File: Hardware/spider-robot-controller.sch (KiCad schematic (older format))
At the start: 27 parts, among them CON1 AVR-ISP-6, CON2 BARREL_JACK, IC1 ATMEGA328-P, P1 SERVO_HEADER, P10 SERVO_HEADER, P11 SERVO_HEADER, P12 SERVO_HEADER, P13 Bluetooth_header, P2 SERVO_HEADER, P3 SERVO_HEADER, P4 SERVO_HEADER, P5 SERVO_HEADER, P6 SERVO_HEADER, P7 SERVO_HEADER, P8 SERVO_HEADER, P9 SERVO_HEADER, SW1 SW_PUSH, U1 LM7805, Y1 16MHz

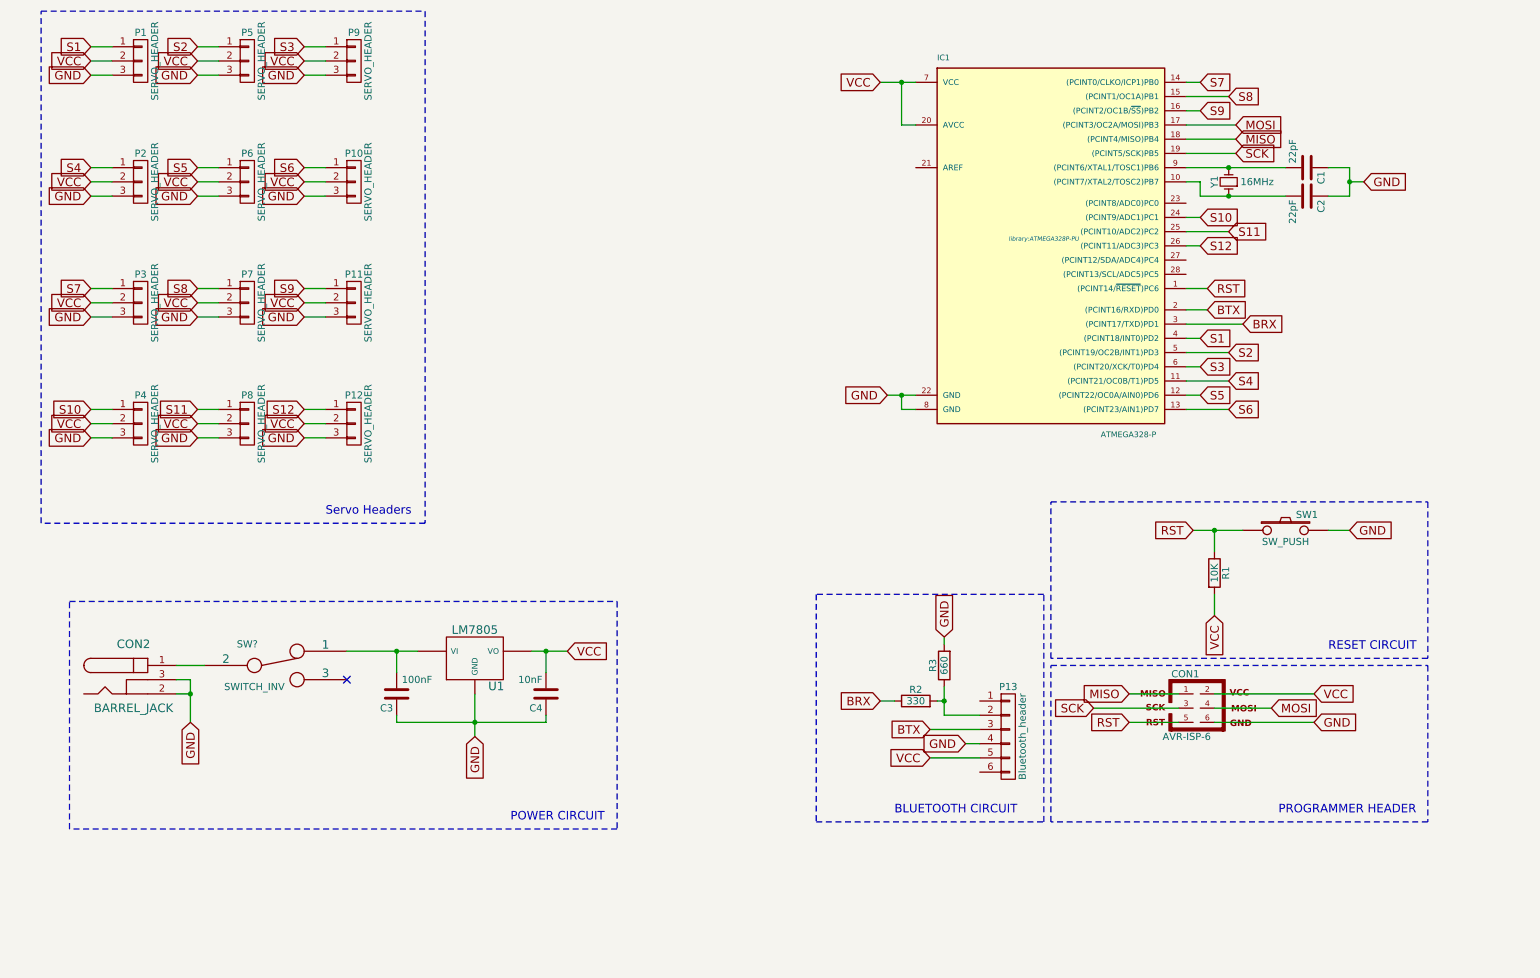
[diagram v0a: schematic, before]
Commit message: working on pcb
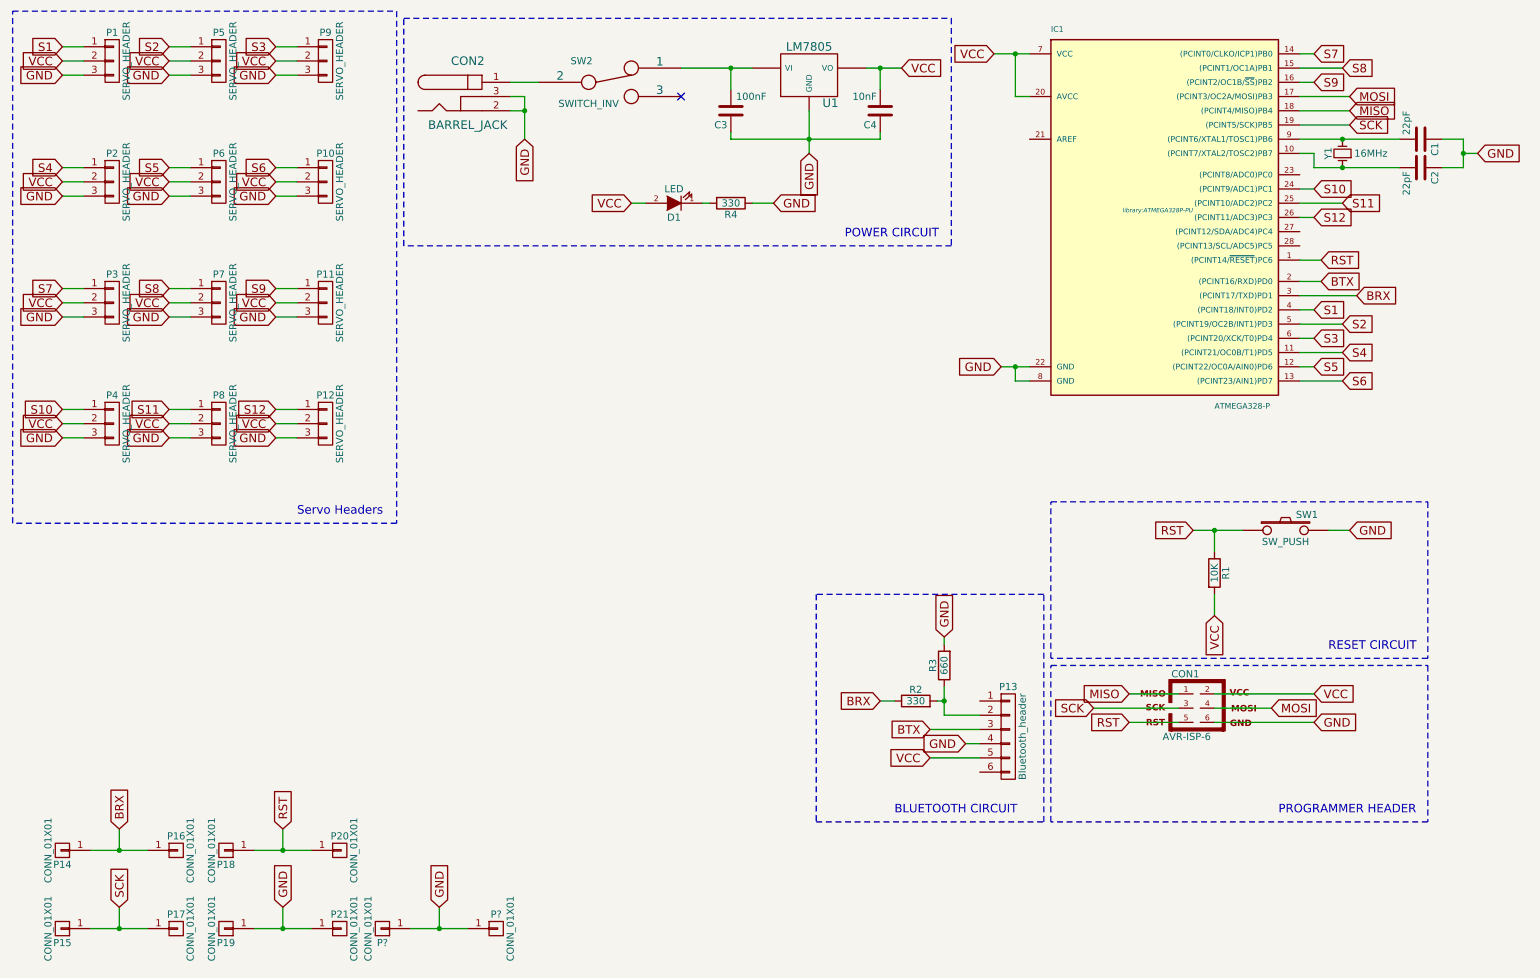
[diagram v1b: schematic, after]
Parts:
- added D1: LED, LEDs:LED-5MM, symbol LED
- added P14, P15, P16, P17, P18, P19, P20, P21, P? (x2): CONN_01X01, Pin_Headers:Pin_Header_Straight_1x01, symbol CONN_01X01
- added R4: 330, Resistors_ThroughHole:Resistor_Horizontal_RM10mm, symbol R
- SW2: renamed from SW?; footprint (none) -> library:SWITCH_INVERTER
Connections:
- net BRX: now also P14.1 (P1), P16.1 (P1)
- net GND: now also P19.1 (P1), P21.1 (P1), P?.1 (P1), P?.1 (P1), R4.1
- net RST: now also P18.1 (P1), P20.1 (P1)
- net SCK: now also P15.1 (P1), P17.1 (P1)
- net VCC: now also D1.2 (A)
- new net: D1.1 (K), R4.2
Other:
- moved on the sheet: C1, C2, C3, C4, CON2, IC1, P1, P10, P11, P12, P2, P3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
